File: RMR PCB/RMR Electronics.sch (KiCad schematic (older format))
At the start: 19 parts, among them J1 Arduino Power, J2 RPI Power, J3 Mast Servo, J4 RMotor, J5 LMotor, J6 Conn_01x01_Male, J7 LMotor Control, J8 RMotor Control, J9 PJ-037A, U1 LD1117S18TR_SOT223, U2 LD1117S18TR_SOT223

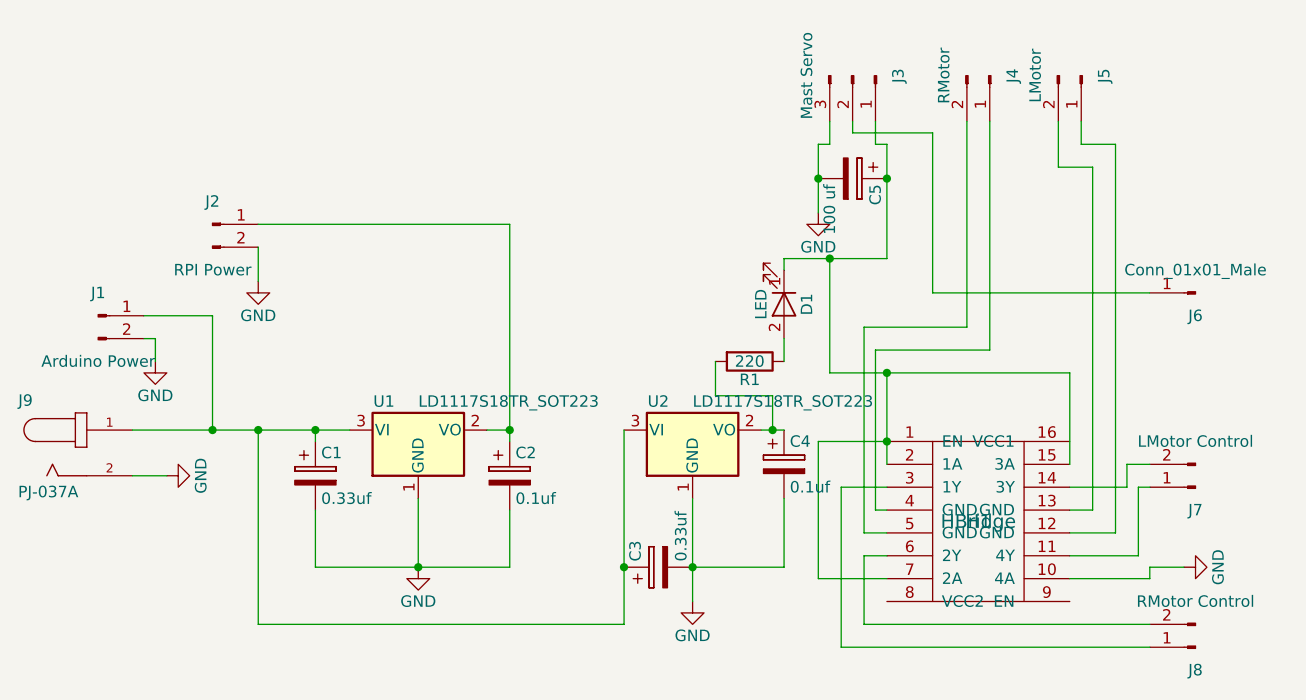
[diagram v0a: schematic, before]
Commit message: started PCB layout
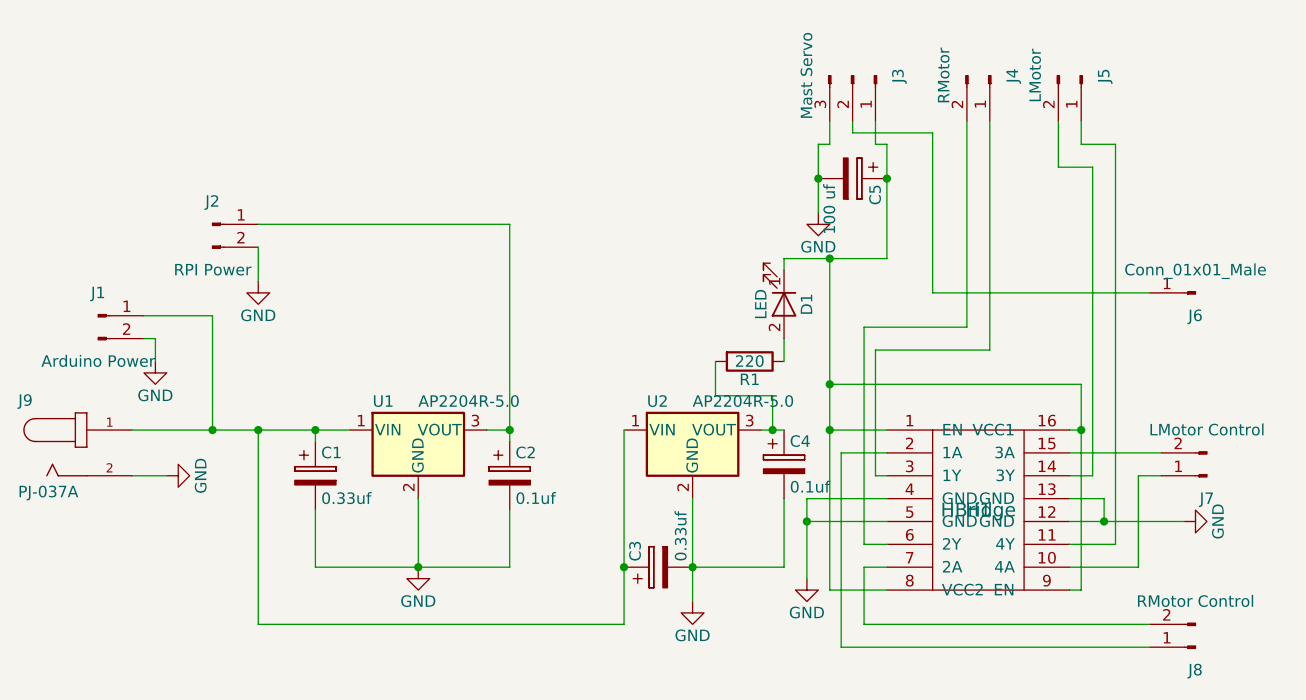
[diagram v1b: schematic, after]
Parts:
- removed U1, U2: LD1117S18TR_SOT223, TO_SOT_Packages_SMD:SOT-223-3Lead_TabPin2, symbol LD1117S18TR_SOT223
- added U1, U2: AP2204R-5.0, TO_SOT_Packages_SMD:SOT-89-3, symbol AP2204R-5.0
- J9: footprint CUI_PJ-037A -> PJ-037A:CUI_PJ-037A
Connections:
- net GND: now also H1.12 (GND), H1.13 (GND), H1.4 (GND), H1.5 (GND), U1.2 (GND), U2.2 (GND); no longer H1.10 (4A)
- net at C2.1, J2.1 (Pin_1): now also U1.3 (VOUT)
- net at C1.1, C3.1, J1.1 (Pin_1)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: now also U1.1 (VIN), U2.1 (VIN)
- net at C4.1, R1.2: now also U2.3 (VOUT)
- net at C5.1, D1.1 (K), H1.1 (EN)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: now also H1.16 (VCC1), H1.8 (VCC2), H1.9 (EN); no longer H1.15 (3A), H1.2 (1A), H1.7 (2A)
- net at J8.1 (Pin_1): now also H1.2 (1A); no longer H1.3 (1Y)
- net at J8.2 (Pin_2): now also H1.7 (2A); no longer H1.6 (2Y)
- net at J7.1 (Pin_1): now also H1.10 (4A); no longer H1.11 (4Y)
- net at J5.1 (Pin_1): now also H1.11 (4Y); no longer H1.12 (GND)
- net at J5.2 (Pin_2): now also H1.14 (3Y); no longer H1.13 (GND)
- net at J7.2 (Pin_2): now also H1.15 (3A); no longer H1.14 (3Y)
- net at J4.1 (Pin_1): now also H1.3 (1Y); no longer H1.4 (GND)
- net at J4.2 (Pin_2): now also H1.6 (2Y); no longer H1.5 (GND)
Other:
- moved on the sheet: H1, J7
